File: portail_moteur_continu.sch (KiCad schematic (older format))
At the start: 84 parts, among them J1 Screw_Terminal_01x02, J10 Conn_01x01_Male, J11 Conn_01x08_Male, J2 Screw_Terminal_01x03, J3 Conn_01x04, J4 Screw_Terminal_01x06, J5 Screw_Terminal_01x03, J6 Conn_01x06_Male, J7 Screw_Terminal_01x02, J8 Conn_01x01_Male, J9 Conn_01x01_Male, K1 FINDER-44.62, Q1 BC548, Q2 BS170, Q3 BS170, U1 SFH617A-1, U2 SFH617A-1, U3 LM7805_TO220, U4 SFH617A-1, U5 SFH617A-1

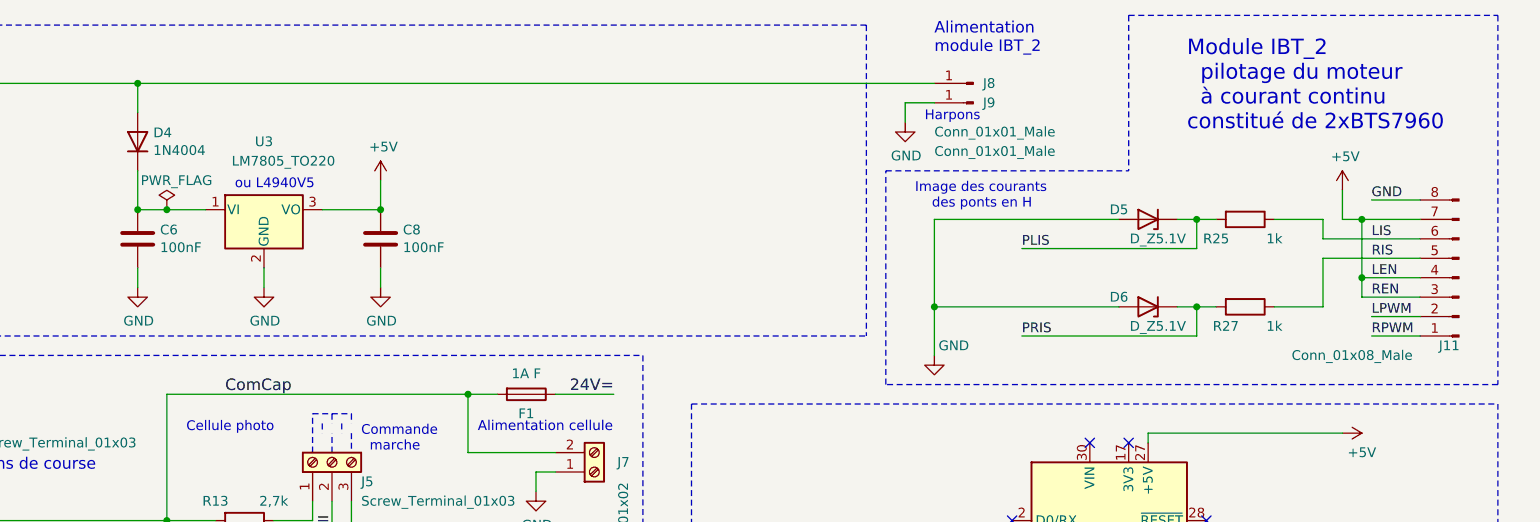
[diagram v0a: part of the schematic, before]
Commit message: V1.1
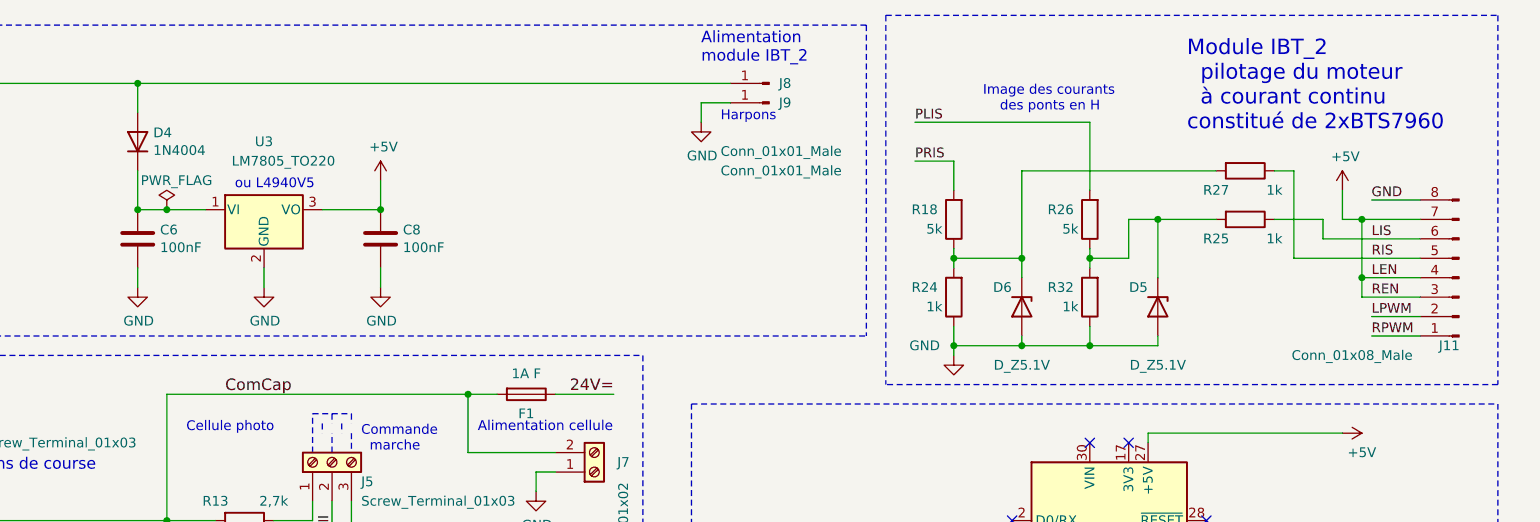
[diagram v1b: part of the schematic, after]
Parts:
- added R18, R26: 5k, Resistor_THT:R_Axial_DIN0207_L6.3mm_D2.5mm_P7.62mm_Horizontal, symbol Device:R
- added R24, R32: 1k, Resistor_THT:R_Axial_DIN0207_L6.3mm_D2.5mm_P7.62mm_Horizontal, symbol Device:R
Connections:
- net GND: now also R24.1, R32.1
- net PLIS: now also R26.2; no longer D5.1 (K), R25.2
- net PRIS: now also R18.2; no longer D6.1 (K), R27.2
- new net: D5.1 (K), R25.2, R26.1, R32.2
- new net: D6.1 (K), R18.1, R24.2, R27.2
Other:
- moved on the sheet: D5, D6, J8, J9, R27
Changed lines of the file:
@@
 Wire Wire Line
 	2300 1350 2300 1300
-Wire Notes Line
-	9200 550  11100 550
 Text Notes 9500 1150 0    79   ~ 0
      Module IBT_2\n  pilotage du moteur \n  à courant continu\nconstitué de 2xBTS7960
-Text Notes 8200 750  0    59   ~ 0
-Alimentation\nmodule IBT_2
-Wire Wire Line
-	8200 1000 8050 1000
-Wire Wire Line
-	8050 1000 8050 1100
-$Comp
-L power:GND #PWR022
-U 1 1 62C27742
-P 8050 1100
-F 0 "#PWR022" H 8050 850 50  0001 C CNN
-F 1 "GND" H 8055 927 50  0000 C CNN
-F 2 "" H 8050 1100 50  0001 C CNN
-F 3 "" H 8050 1100 50  0001 C CNN
-	1    8050 1100
-	1    0    0    -1
-$EndComp
 $Comp
 L Connector:Conn_01x08_Male J11
@@
 GND
 $Comp
-L power:GND #PWR023
-U 1 1 62C0D486
-P 8200 2300
-F 0 "#PWR023" H 8200 2050 50  0001 C CNN
-F 1 "GND" H 8300 2350 50  0000 C CNN
-F 2 "" H 8200 2300 50  0001 C CNN
-F 3 "" H 8200 2300 50  0001 C CNN
-	1    8200 2300
-	1    0    0    -1
-$EndComp
-$Comp
 L Device:D_Zener D5
 U 1 1 62C5A5F0
-P 9300 1600
-F 0 "D5" H 9450 1550 50  0000 C CNN
-F 1 "D_Z5.1V" H 9250 1700 50  0000 C CNN
-F 2 "Diode_THT:D_A-405_P7.62mm_Horizontal" H 9300 1600 50  0001 C CNN
-F 3 "~" H 9300 1600 50  0001 C CNN
-	1    9300 1600
-	-1   0    0    1
+P 9350 2050
+F 0 "D5" V 9250 1950 50  0000 C CNN
+F 1 "D_Z5.1V" V 9650 2050 50  0000 C CNN
+F 2 "Diode_THT:D_A-405_P7.62mm_Horizontal" H 9350 2050 50  0001 C CNN
+F 3 "~" H 9350 2050 50  0001 C CNN
+	1    9350 2050
+	0    1    1    0
 $EndComp
 $Comp
@@
 	0    1    1    0
 $EndComp
-Wire Wire Line
-	9450 1600 9550 1600
-Wire Wire Line
-	9550 1600 9550 1750
-Connection ~ 9550 1600
-Wire Wire Line
-	9550 1600 9650 1600
 $Comp
 L Device:D_Zener D6
 U 1 1 62C71CA2
-P 9300 2050
-F 0 "D6" H 9450 2000 50  0000 C CNN
-F 1 "D_Z5.1V" H 9250 2150 50  0000 C CNN
-F 2 "Diode_THT:D_A-405_P7.62mm_Horizontal" H 9300 2050 50  0001 C CNN
-F 3 "~" H 9300 2050 50  0001 C CNN
-	1    9300 2050
-	-1   0    0    1
+P 8650 2050
+F 0 "D6" V 8550 1950 50  0000 C CNN
+F 1 "D_Z5.1V" V 8950 2050 50  0000 C CNN
+F 2 "Diode_THT:D_A-405_P7.62mm_Horizontal" H 8650 2050 50  0001 C CNN
+F 3 "~" H 8650 2050 50  0001 C CNN
+	1    8650 2050
+	0    1    1    0
 $EndComp
 $Comp
 L Device:R R27
 U 1 1 62C71CAC
-P 9800 2050
-F 0 "R27" V 9900 1950 50  0000 C CNN
-F 1 "1k" V 9900 2200 50  0000 C CNN
-F 2 "Resistor_THT:R_Axial_DIN0207_L6.3mm_D2.5mm_P7.62mm_Horizontal" V 9730 2050 50  0001 C CNN
-F 3 "~" H 9800 2050 50  0001 C CNN
-	1    9800 2050
-	0    1    1    0
-$EndComp
-Wire Wire Line
-	9450 2050 9550 2050
-Wire Wire Line
-	9550 2050 9550 2200
-Connection ~ 9550 2050
-Wire Wire Line
-	9550 2050 9650 2050
-Text Label 8650 1750 0    50   ~ 0
-PLIS
-Text Label 8650 2200 0    50   ~ 0
-PRIS
-Wire Wire Line
-	9550 2200 8650 2200
+P 9800 1350
+F 0 "R27" V 9900 1200 50  0000 C CNN
+F 1 "1k" V 9900 1500 50  0000 C CNN
+F 2 "Resistor_THT:R_Axial_DIN0207_L6.3mm_D2.5mm_P7.62mm_Horizontal" V 9730 1350 50  0001 C CNN
+F 3 "~" H 9800 1350 50  0001 C CNN
+	1    9800 1350
+	0    1    1    0
+$EndComp
 $Comp
 L power:+5V #PWR017
@@
 Text Label 4650 4300 1    50   ~ 0
 Ferme
-Wire Wire Line
-	9550 1750 8650 1750
 Wire Notes Line
 	550  2300 2500 2300
@@
 	10200 1700 10200 1600
 Wire Wire Line
-	10700 1800 10200 1800
-Wire Wire Line
 	9950 1600 10200 1600
-Wire Wire Line
-	9950 2050 10200 2050
 $Comp
 L Relay:FINDER-44.62 K1
@@
 Wire Wire Line
 	10450 4050 10800 4050
-Text Notes 8100 1550 0    50   ~ 0
+Text Notes 8450 1050 0    50   ~ 0
 Image des courants\n    des ponts en H
 $Comp
@@
 $EndComp
 $Comp
-L Connector:Conn_01x01_Male J8
-U 1 1 62CD651F
-P 8400 900
-F 0 "J8" H 8350 900 50  0000 R CNN
-F 1 "Conn_01x01_Male" H 8600 1250 50  0000 R CNN
-F 2 "Connector_PinHeader_2.54mm:PinHeader_1x01_P2.54mm_Vertical" H 8400 900 50  0001 C CNN
-F 3 "~" H 8400 900 50  0001 C CNN
-	1    8400 900
-	-1   0    0    1
-$EndComp
-$Comp
-L Connector:Conn_01x01_Male J9
-U 1 1 62CD72A3
-P 8400 1000
-F 0 "J9" H 8350 1000 50  0000 R CNN
-F 1 "Conn_01x01_Male" H 8600 1150 50  0000 R CNN
-F 2 "Connector_PinHeader_2.54mm:PinHeader_1x01_P2.54mm_Vertical" H 8400 1000 50  0001 C CNN
-F 3 "~" H 8400 1000 50  0001 C CNN
-	1    8400 1000
-	-1   0    0    1
-$EndComp
-Text Notes 8150 1100 0    50   ~ 0
-Harpons
-$Comp
 L Mechanical:Fiducial FID9
 U 1 1 62C96000
@@
 	9200 4800 9200 4750
 Wire Notes Line
-	9200 550  9200 1350
-Wire Notes Line
 	11100 550  11100 2450
 Wire Notes Line
@@
 Wire Notes Line
 	6950 2550 11100 2550
-Wire Notes Line
-	7950 2450 7950 1350
-Wire Notes Line
-	7950 1350 9200 1350
 Wire Notes Line
 	11100 2450 7950 2450
@@
 Wire Notes Line
 	2500 2300 2500 5400
-Connection ~ 4100 900
 Wire Wire Line
 	6000 3850 6000 3950
@@
 	0    1    1    0
 $EndComp
-Wire Wire Line
-	2850 900  4100 900
 NoConn ~ 8600 3350
 NoConn ~ 8600 3250
@@
 Text Notes 1900 7250 0    59   ~ 0
 ou BC546,\nBC547, \nBC548,\nBC549,\nBC550
-Wire Wire Line
-	8200 2050 8200 2300
-Wire Wire Line
-	8200 1600 8200 2050
-Connection ~ 8200 2050
-Wire Wire Line
-	4100 900  8200 900
 Wire Wire Line
 	6250 2500 6550 2500
@@
 Wire Notes Line style solid
 	3200 2800 3200 2600
-Wire Wire Line
-	8200 1600 9150 1600
-Wire Wire Line
-	10200 1800 10200 2050
-Wire Wire Line
-	8200 2050 9150 2050
 $Comp
 L power:GND #PWR0101
@@
 Wire Wire Line
 	5050 1550 5350 1550
+Connection ~ 4100 900
+Text Notes 7100 1100 0    50   ~ 0
+Harpons
+$Comp
+L Connector:Conn_01x01_Male J9
+U 1 1 62CD72A3
+P 7350 1000
+F 0 "J9" H 7300 1000 50  0000 R CNN
+F 1 "Conn_01x01_Male" H 7600 1250 50  0000 R CNN
+F 2 "Connector_PinHeader_2.54mm:PinHeader_1x01_P2.54mm_Vertical" H 7350 1000 50  0001 C CNN
+F 3 "~" H 7350 1000 50  0001 C CNN
+	1    7350 1000
+	-1   0    0    1
+$EndComp
+$Comp
+L Connector:Conn_01x01_Male J8
+U 1 1 62CD651F
+P 7350 900
+F 0 "J8" H 7300 900 50  0000 R CNN
+F 1 "Conn_01x01_Male" H 7600 1350 50  0000 R CNN
+F 2 "Connector_PinHeader_2.54mm:PinHeader_1x01_P2.54mm_Vertical" H 7350 900 50  0001 C CNN
+F 3 "~" H 7350 900 50  0001 C CNN
+	1    7350 900
+	-1   0    0    1
+$EndComp
+$Comp
+L power:GND #PWR022
+U 1 1 62C27742
+P 7000 1100
+F 0 "#PWR022" H 7000 850 50  0001 C CNN
+F 1 "GND" H 7005 927 50  0000 C CNN
+F 2 "" H 7000 1100 50  0001 C CNN
+F 3 "" H 7000 1100 50  0001 C CNN
+	1    7000 1100
+	1    0    0    -1
+$EndComp
+Wire Wire Line
+	7000 1000 7000 1100
+Wire Wire Line
+	7150 1000 7000 1000
+Text Notes 7000 800  0    59   ~ 0
+Alimentation\nmodule IBT_2
+Wire Wire Line
+	4100 900  7150 900
+Wire Wire Line
+	2850 900  4100 900
+Wire Notes Line
+	7950 550  11100 550
+Wire Notes Line
+	7950 550  7950 2450
+Text Label 8100 1300 0    50   ~ 0
+PRIS
+Text Label 8100 1100 0    50   ~ 0
+PLIS
+$Comp
+L Device:R R26
+U 1 1 6310F759
+P 9000 1600
+F 0 "R26" H 9150 1550 50  0000 C CNN
+F 1 "5k" H 9100 1650 50  0000 C CNN
+F 2 "Resistor_THT:R_Axial_DIN0207_L6.3mm_D2.5mm_P7.62mm_Horizontal" V 8930 1600 50  0001 C CNN
+F 3 "~" H 9000 1600 50  0001 C CNN
+	1    9000 1600
+	-1   0    0    1
+$EndComp
+$Comp
+L Device:R R32
+U 1 1 631278AE
+P 9000 2000
+F 0 "R32" H 9150 1950 50  0000 C CNN
+F 1 "1k" H 9100 2050 50  0000 C CNN
+F 2 "Resistor_THT:R_Axial_DIN0207_L6.3mm_D2.5mm_P7.62mm_Horizontal" V 8930 2000 50  0001 C CNN
+F 3 "~" H 9000 2000 50  0001 C CNN
+	1    9000 2000
+	-1   0    0    1
+$EndComp
+$Comp
+L Device:R R18
+U 1 1 631C9841
+P 8300 1600
+F 0 "R18" H 8450 1550 50  0000 C CNN
+F 1 "5k" H 8400 1650 50  0000 C CNN
+F 2 "Resistor_THT:R_Axial_DIN0207_L6.3mm_D2.5mm_P7.62mm_Horizontal" V 8230 1600 50  0001 C CNN
+F 3 "~" H 8300 1600 50  0001 C CNN
+	1    8300 1600
+	-1   0    0    1
+$EndComp
+$Comp
+L Device:R R24
+U 1 1 631C9848
+P 8300 2000
+F 0 "R24" H 8450 1950 50  0000 C CNN
+F 1 "1k" H 8400 2050 50  0000 C CNN
+F 2 "Resistor_THT:R_Axial_DIN0207_L6.3mm_D2.5mm_P7.62mm_Horizontal" V 8230 2000 50  0001 C CNN
+F 3 "~" H 8300 2000 50  0001 C CNN
+	1    8300 2000
+	-1   0    0    1
+$EndComp
+Wire Wire Line
+	8300 1750 8300 1800
+Connection ~ 8300 1800
+Wire Wire Line
+	8300 1800 8300 1850
+$Comp
+L power:GND #PWR023
+U 1 1 6327580F
+P 8300 2300
+F 0 "#PWR023" H 8300 2050 50  0001 C CNN
+F 1 "GND" H 8150 2350 50  0000 C CNN
+F 2 "" H 8300 2300 50  0001 C CNN
+F 3 "" H 8300 2300 50  0001 C CNN
+	1    8300 2300
+	1    0    0    -1
+$EndComp
+Wire Wire Line
+	8300 1300 8100 1300
+Wire Wire Line
+	8300 1300 8300 1450
+Wire Wire Line
+	8100 1100 9000 1100
+Wire Wire Line
+	8650 1800 8650 1900
+Wire Wire Line
+	8300 1800 8650 1800
+Wire Wire Line
+	8300 2150 8300 2250
+Wire Wire Line
+	8650 2200 8650 2250
+Wire Wire Line
+	8650 2250 8300 2250
+Connection ~ 8300 2250
+Wire Wire Line
+	8300 2250 8300 2300
+Wire Wire Line
+	8650 2250 9000 2250
+Connection ~ 8650 2250
+Wire Wire Line
+	9000 2150 9000 2250
+Wire Wire Line
+	9000 1750 9000 1800
+Wire Wire Line
+	9000 1800 9200 1800
+Wire Wire Line
+	9200 1800 9200 1600
+Connection ~ 9000 1800
+Wire Wire Line
+	9000 1800 9000 1850
+Wire Wire Line
+	9000 2250 9350 2250
+Connection ~ 9000 2250
+Wire Wire Line
+	9000 1100 9000 1450
+Wire Wire Line
+	10050 1350 9950 1350
+Wire Wire Line
+	10050 1800 10050 1350
+Wire Wire Line
+	9650 1350 8650 1350
+Wire Wire Line
+	8650 1350 8650 1800
+Connection ~ 8650 1800
+Wire Wire Line
+	10050 1800 10700 1800
+Wire Wire Line
+	9200 1600 9350 1600
+Wire Wire Line
+	9350 2200 9350 2250
+Wire Wire Line
+	9350 1900 9350 1600
+Connection ~ 9350 1600
+Wire Wire Line
+	9350 1600 9650 1600
 $EndSCHEMATC
